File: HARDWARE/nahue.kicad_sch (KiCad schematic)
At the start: 42 parts, among them J2 Screw_Terminal_01x03, J4 Screw_Terminal_01x03, J5 Screw_Terminal_01x03, J6 Conn_01x08, K1 RELAY, K2 RELAY, K3 RELAY, K4 RELAY, Q1 MMBT3904, Q2 MMBT3904, Q3 MMBT3904, Q4 MMBT3904, U1 PC817, U2 PC817, U3 PC817, U4 PC817, U6 LM7805_TO220

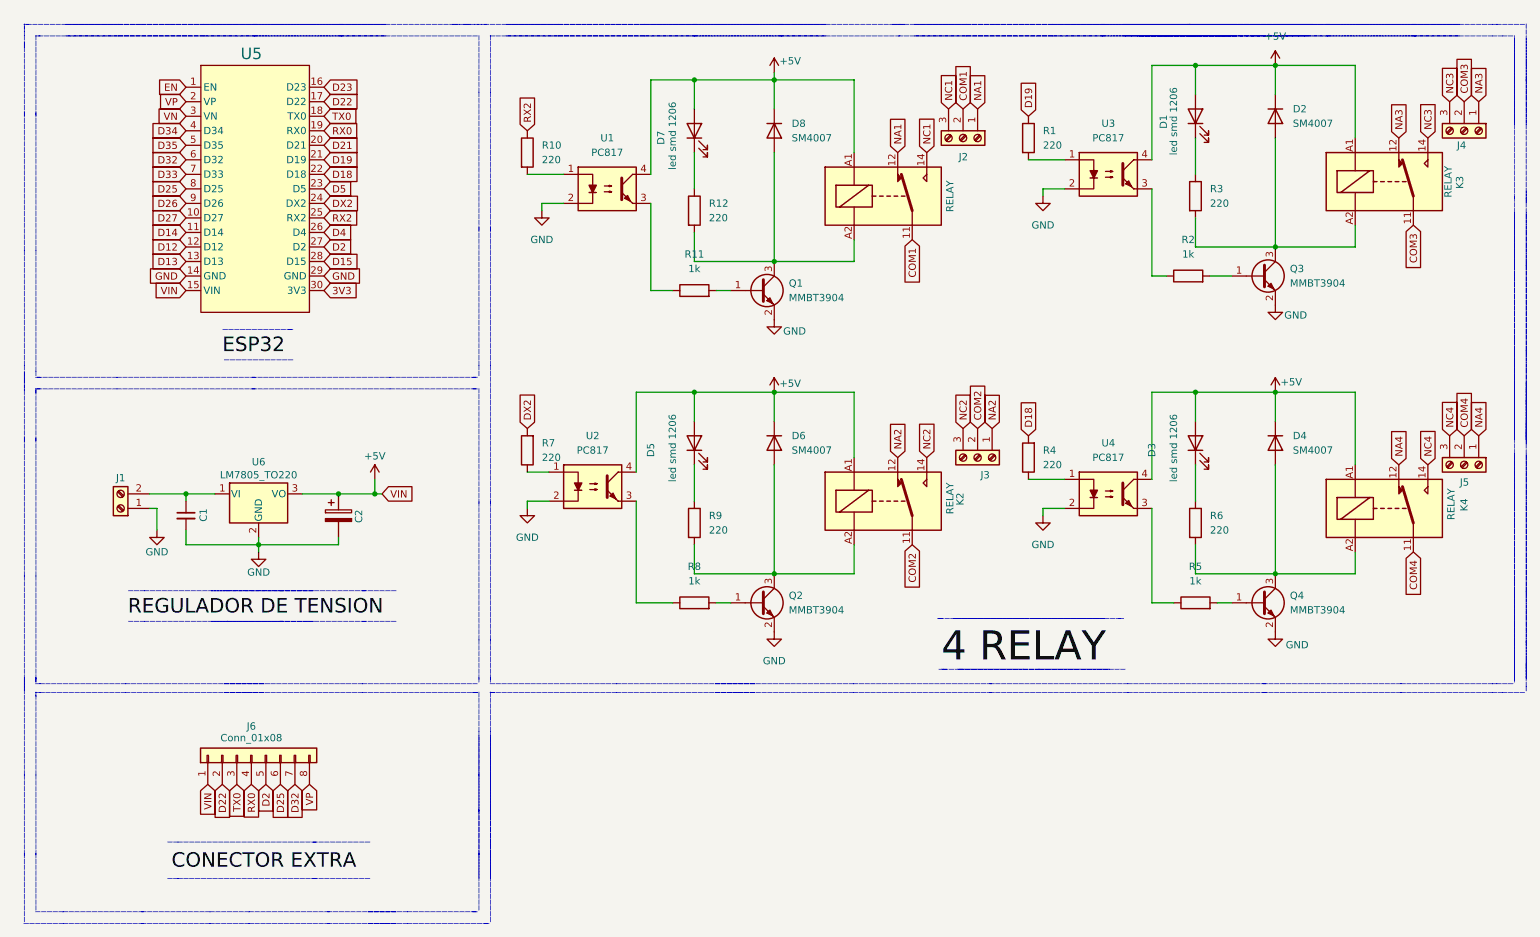
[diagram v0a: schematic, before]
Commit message: finalizado 2
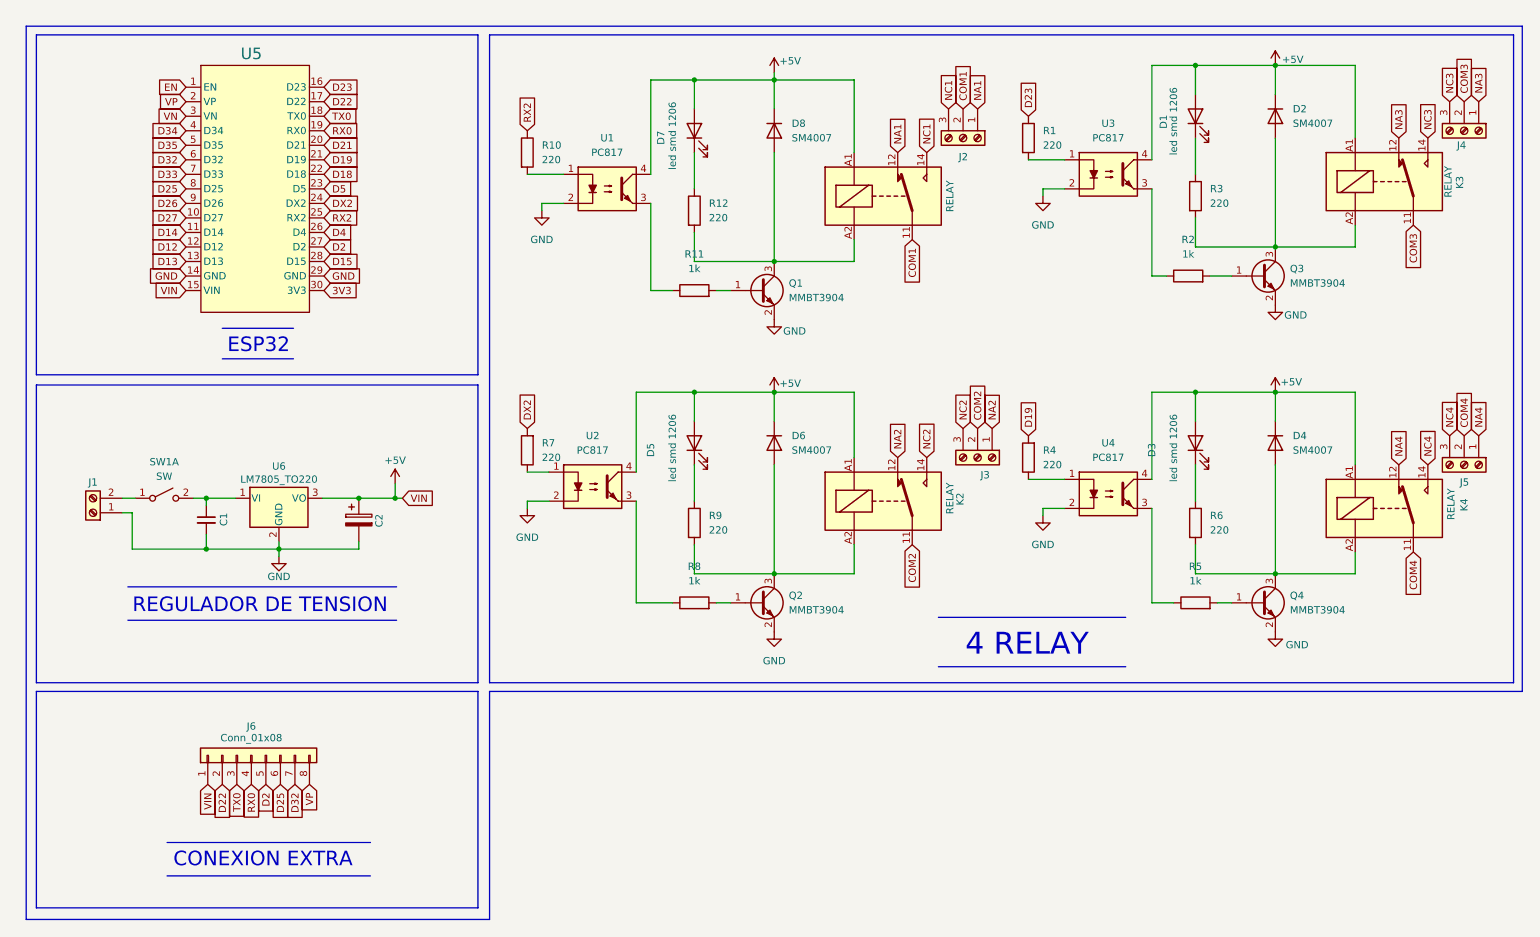
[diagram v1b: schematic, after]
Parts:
- added SW1: SW, Connector_PinHeader_2.54mm:PinHeader_1x02_P2.54mm_Vertical, symbol Switch:SW_DPST_x2
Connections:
- net D18: no longer R4.2
- net D19: now also R4.2; no longer R1.1
- net D23: now also R1.1
- net at C1.1, U6.1 (VI): now also SW1.2 (B); no longer J1.2 (Pin_2)
- new net: J1.2 (Pin_2), SW1.1 (A)
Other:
- note added: "4 RELAY"
- note added: "CONEXION EXTRA"
- note added: "ESP32"
- note added: "REGULADOR DE TENSION"
- note removed: "_"
- moved on the sheet: C1, C2, J1, U6
